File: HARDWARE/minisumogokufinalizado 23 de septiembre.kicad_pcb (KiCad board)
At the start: 2 copper layers, 74.7 x 54 mm, 17 parts, among them J1 batterly, J2 hc-sr05, J3 sensor, M1 Motor_DC, M2 Motor_DC, SW1 SW_DPST_x2, U1 L293D, U2 L7805

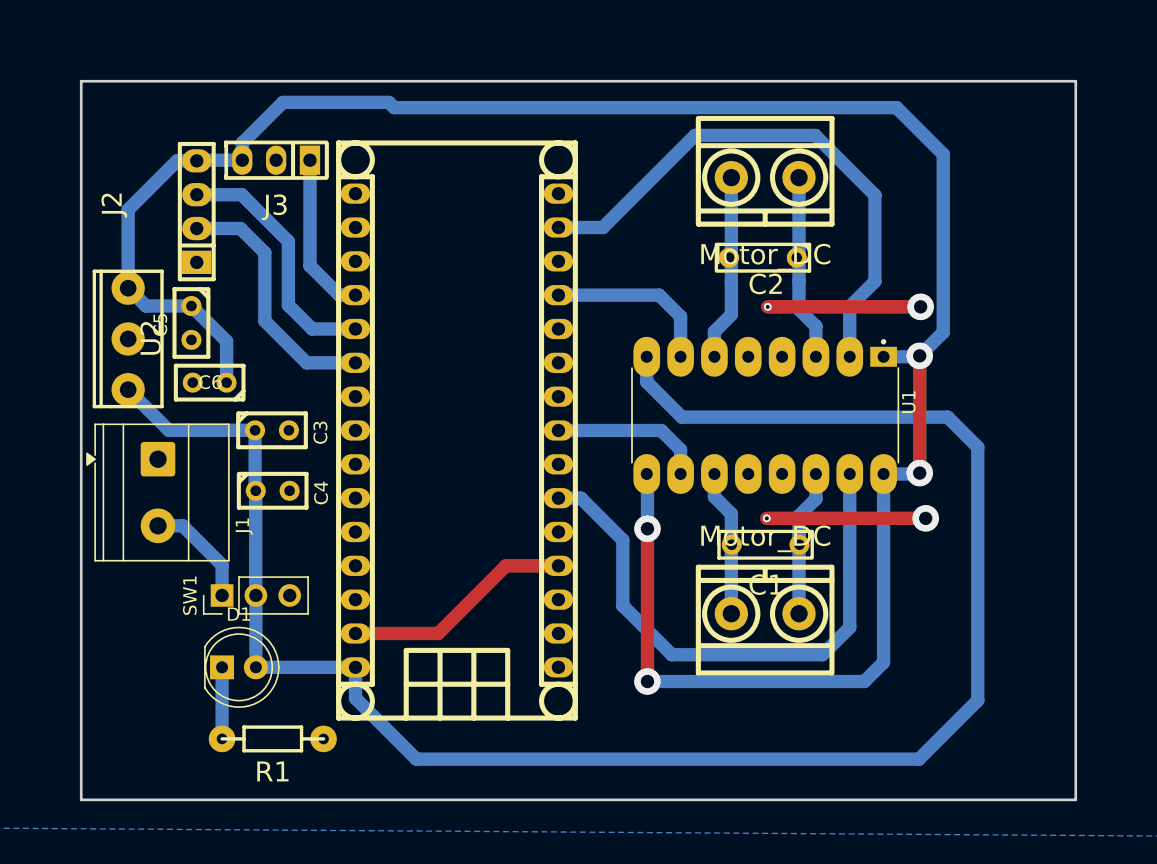
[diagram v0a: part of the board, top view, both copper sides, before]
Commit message: Add files via upload
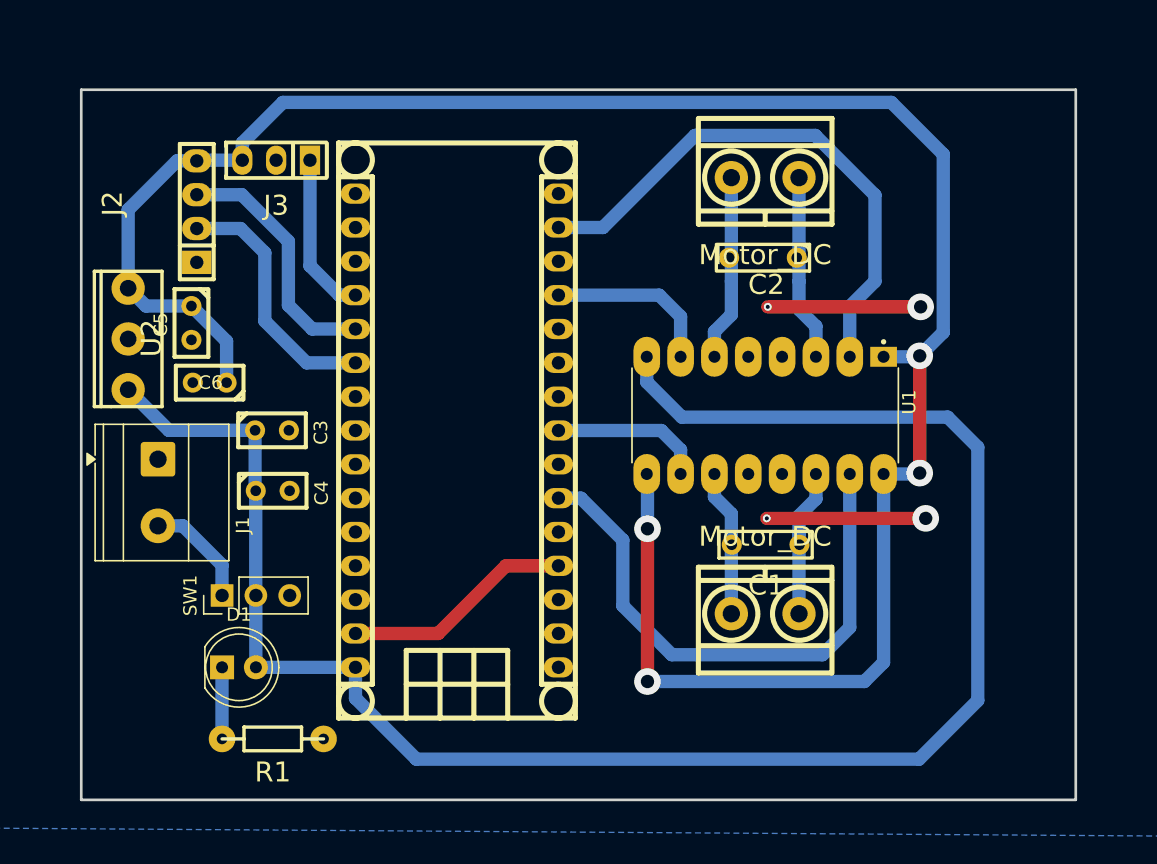
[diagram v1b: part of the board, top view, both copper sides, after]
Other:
- board size 74.7 x 54 mm -> 74.7 x 53.3 mm
